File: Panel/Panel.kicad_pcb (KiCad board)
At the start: 2 copper layers, 30 x 128.5 mm, 6 parts

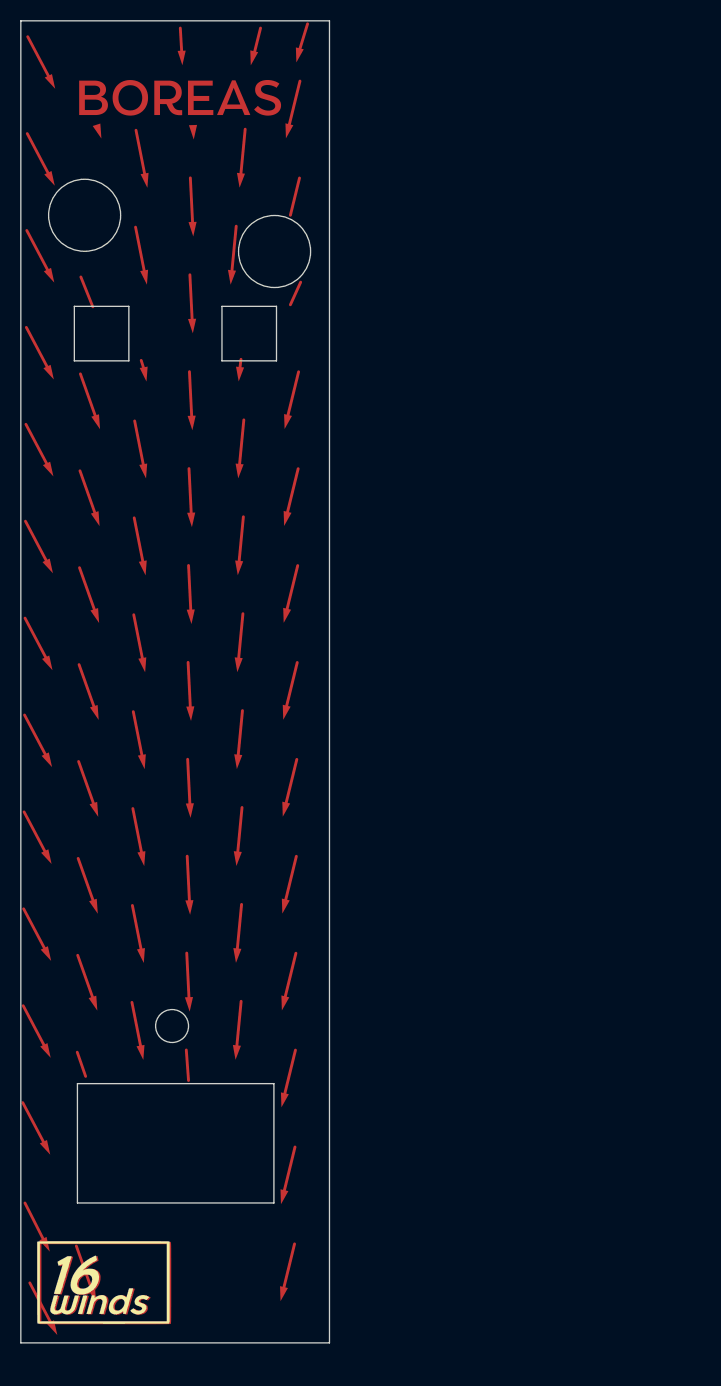
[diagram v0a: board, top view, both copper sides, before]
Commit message: v3.1
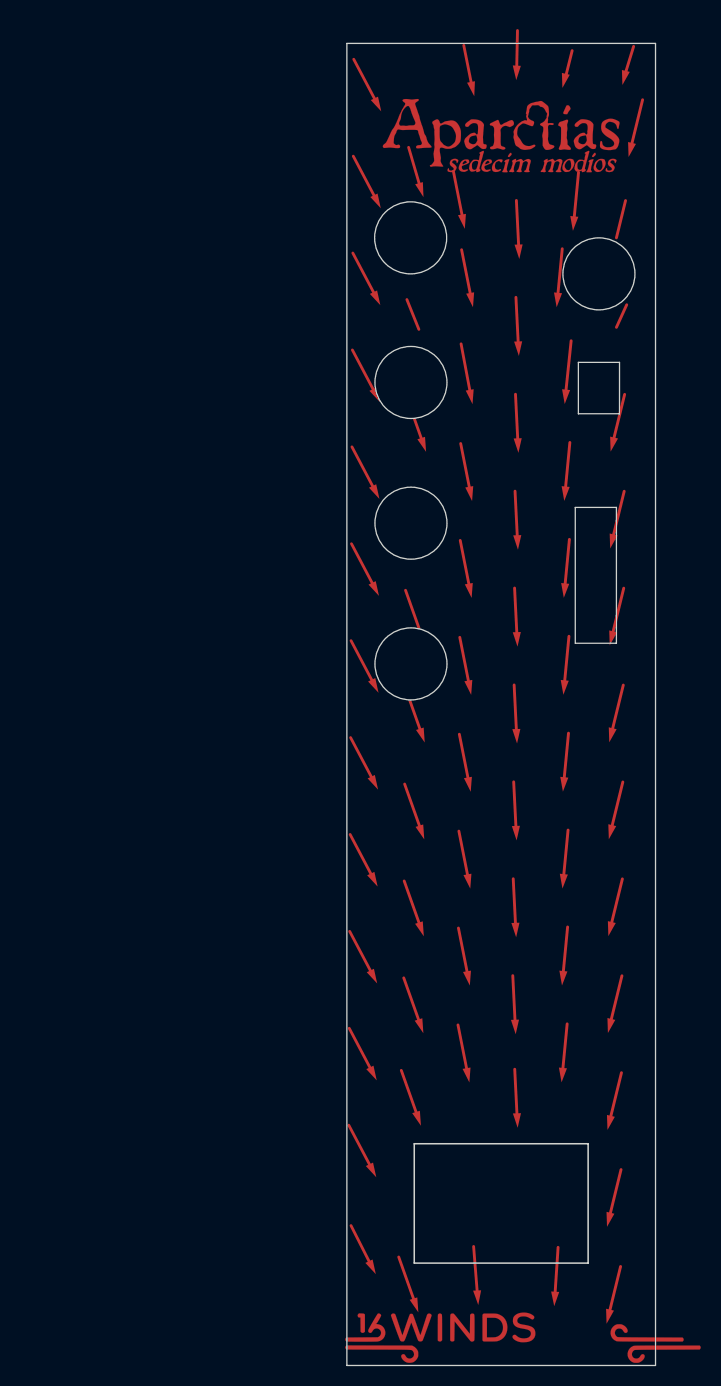
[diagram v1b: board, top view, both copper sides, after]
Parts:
- removed the ? at (59.6, 132.2)
- removed the ? at (67.4, 160.0)
- removed the REF** at (69.5, 56.9)
- removed the REF** at (52.4, 37.5)
- removed the REF** at (51.1, 53.4)
- removed the Ref** at (53.6, 160.5)
- added ?: , , F.Cu at (82.8, 97.0)
- added ?: , , F.Cu at (99.1, 162.2)
- added ?: , , F.Cu at (82.8, 83.3)
- added REF**: MountingHole, MountingHole:MountingHole_3.2mm_M3, F.Cu at (82.8, 69.6)
- added REF**: MountingHole_3.2mm_M3, MountingHole:MountingHole_3.2mm_M3, F.Cu at (84.1, 39.7)
- added REF**: MountingHole, MountingHole:MountingHole_3.2mm_M3, F.Cu at (101.1, 59.1)
- added REF**: MountingHole, MountingHole:MountingHole_3.2mm_M3, F.Cu at (82.8, 55.6)
- added Ref**: Val**, LogoFootprints:sedecim-modios-humane-jenson, F.Cu at (98.7, 51.3)
- added Ref**: Val**, LogoFootprints:16WindsLogoJuly2023-12mm-RightSide, F.Cu at (122.1, 164.6)
- added Ref**: Val**, LogoFootprints:aparticas-glyphs-humane-jenson, F.Cu at (92.2, 46.9)
- added Ref**: Val**, LogoFootprints:16WindsLogoJuly2023-12mm, F.Cu at (96.3, 164.6)
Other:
- outline, holes or cut-outs redrawn
